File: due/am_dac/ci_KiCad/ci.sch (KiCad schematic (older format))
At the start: 8 parts

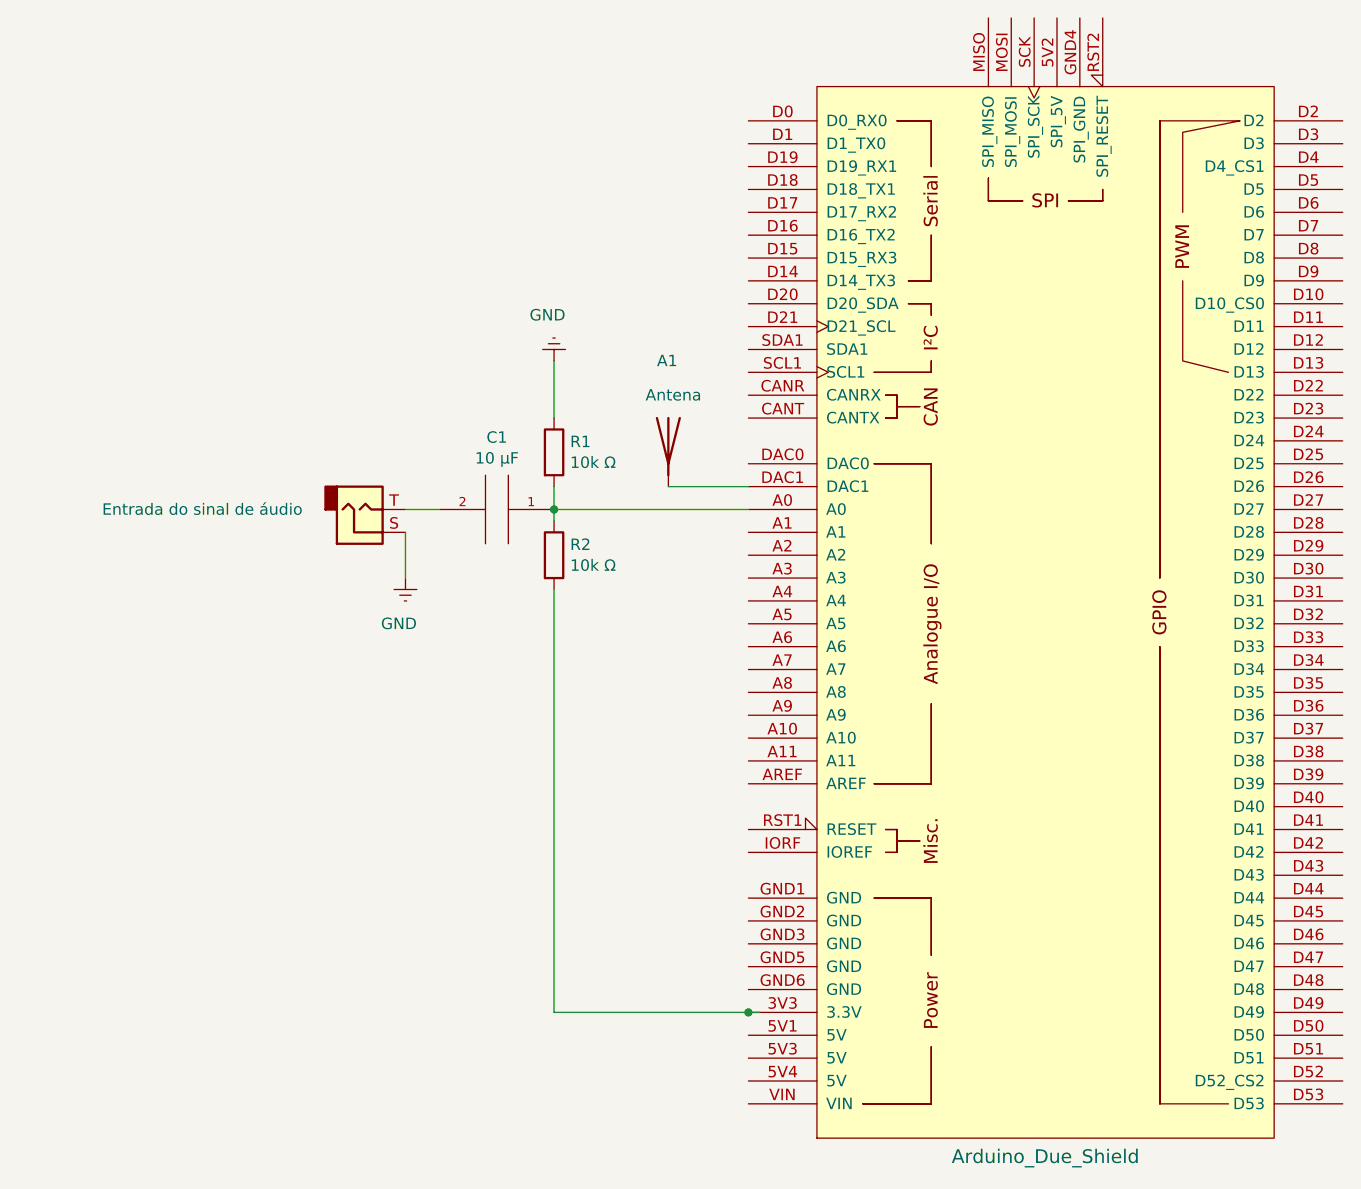
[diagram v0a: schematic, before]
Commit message: Update due am_dac project
Signed-off-by: fgl27 <fglfgl27@gmail.com>
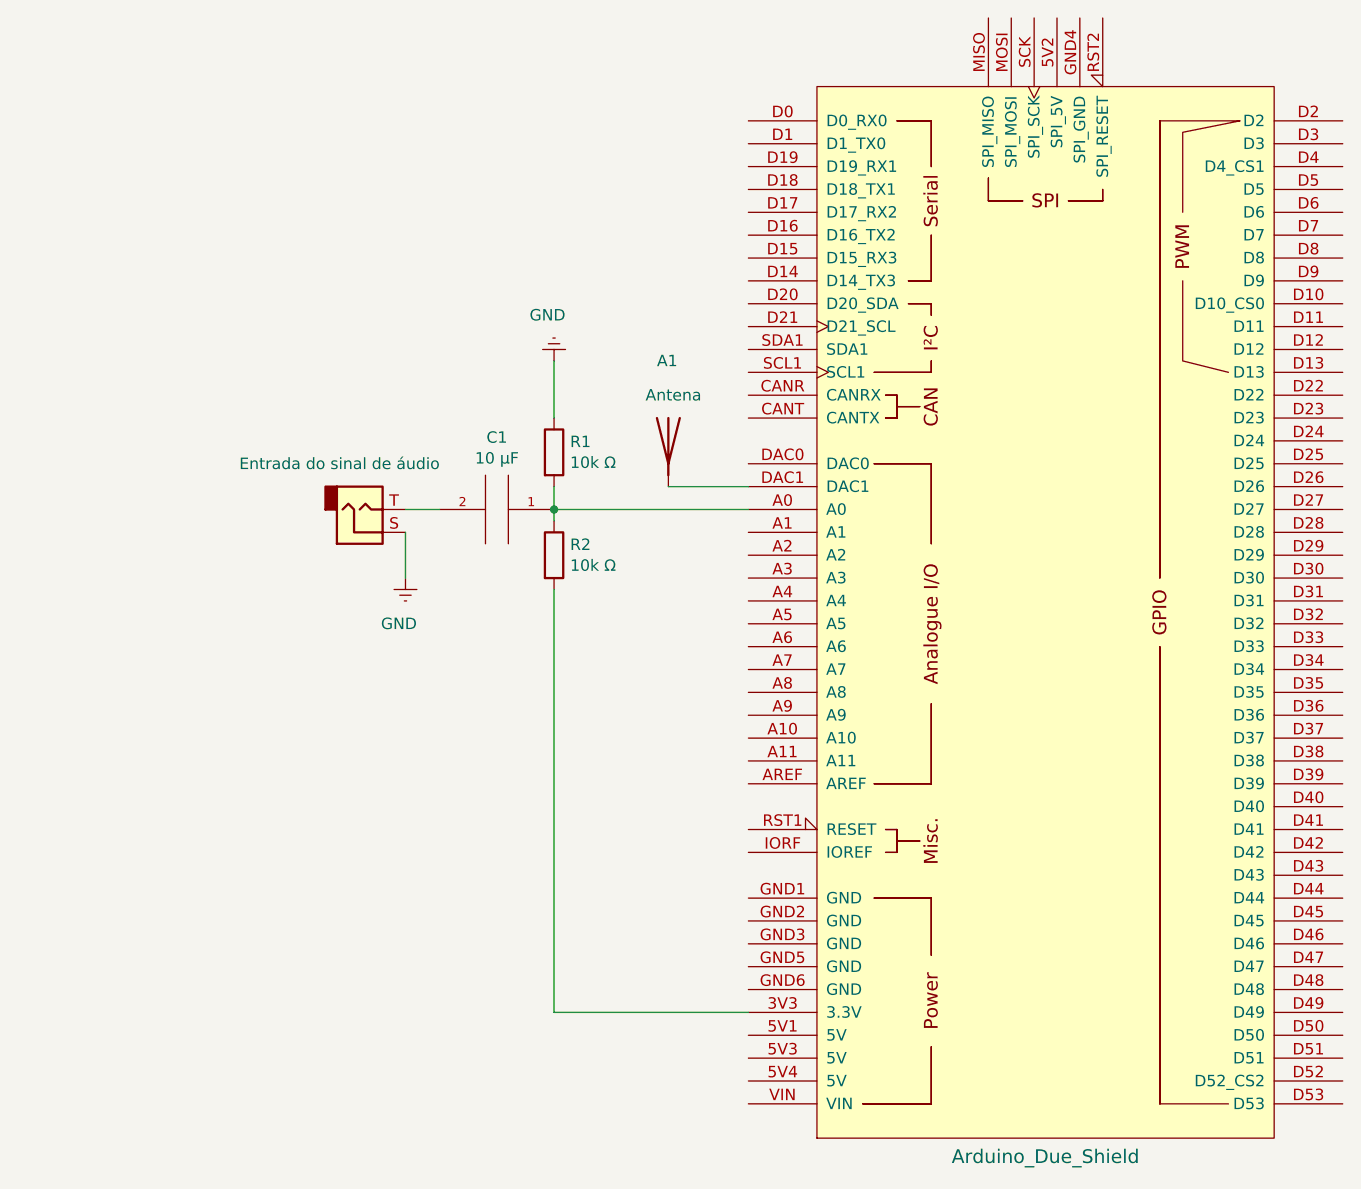
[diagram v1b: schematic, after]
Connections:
- wire segments 10 -> 9
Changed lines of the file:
@@
 P 2600 3250
 F 0 "J?" V 2678 3120 50  0001 R CNN
-F 1 "Entrada do sinal de áudio" H 2350 3250 50  0000 R CNN
+F 1 "Entrada do sinal de áudio" H 2950 3050 50  0000 R CNN
 F 2 "" H 2600 3250 50  0001 C CNN
 F 3 "~" H 2600 3250 50  0001 C CNN
@@
 Wire Wire Line
 	3450 2850 3450 2600
+Wire Wire Line
+	3950 3150 4300 3150
+Wire Wire Line
+	3450 5450 3450 3600
+Wire Wire Line
+	3450 3250 4300 3250
 $Comp
 L arduino:Arduino_Due_Shield XA1
@@
 $EndComp
 Wire Wire Line
-	3950 3150 4300 3150
-Wire Wire Line
-	3450 3250 4300 3250
-Wire Wire Line
-	4350 5450 4300 5450
-Wire Wire Line
-	3450 5450 3450 3600
-Connection ~ 4300 5450
-Wire Wire Line
 	4300 5450 3450 5450

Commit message: Up due am_dac
Signed-off-by: fgl27 <fglfgl27@gmail.com>
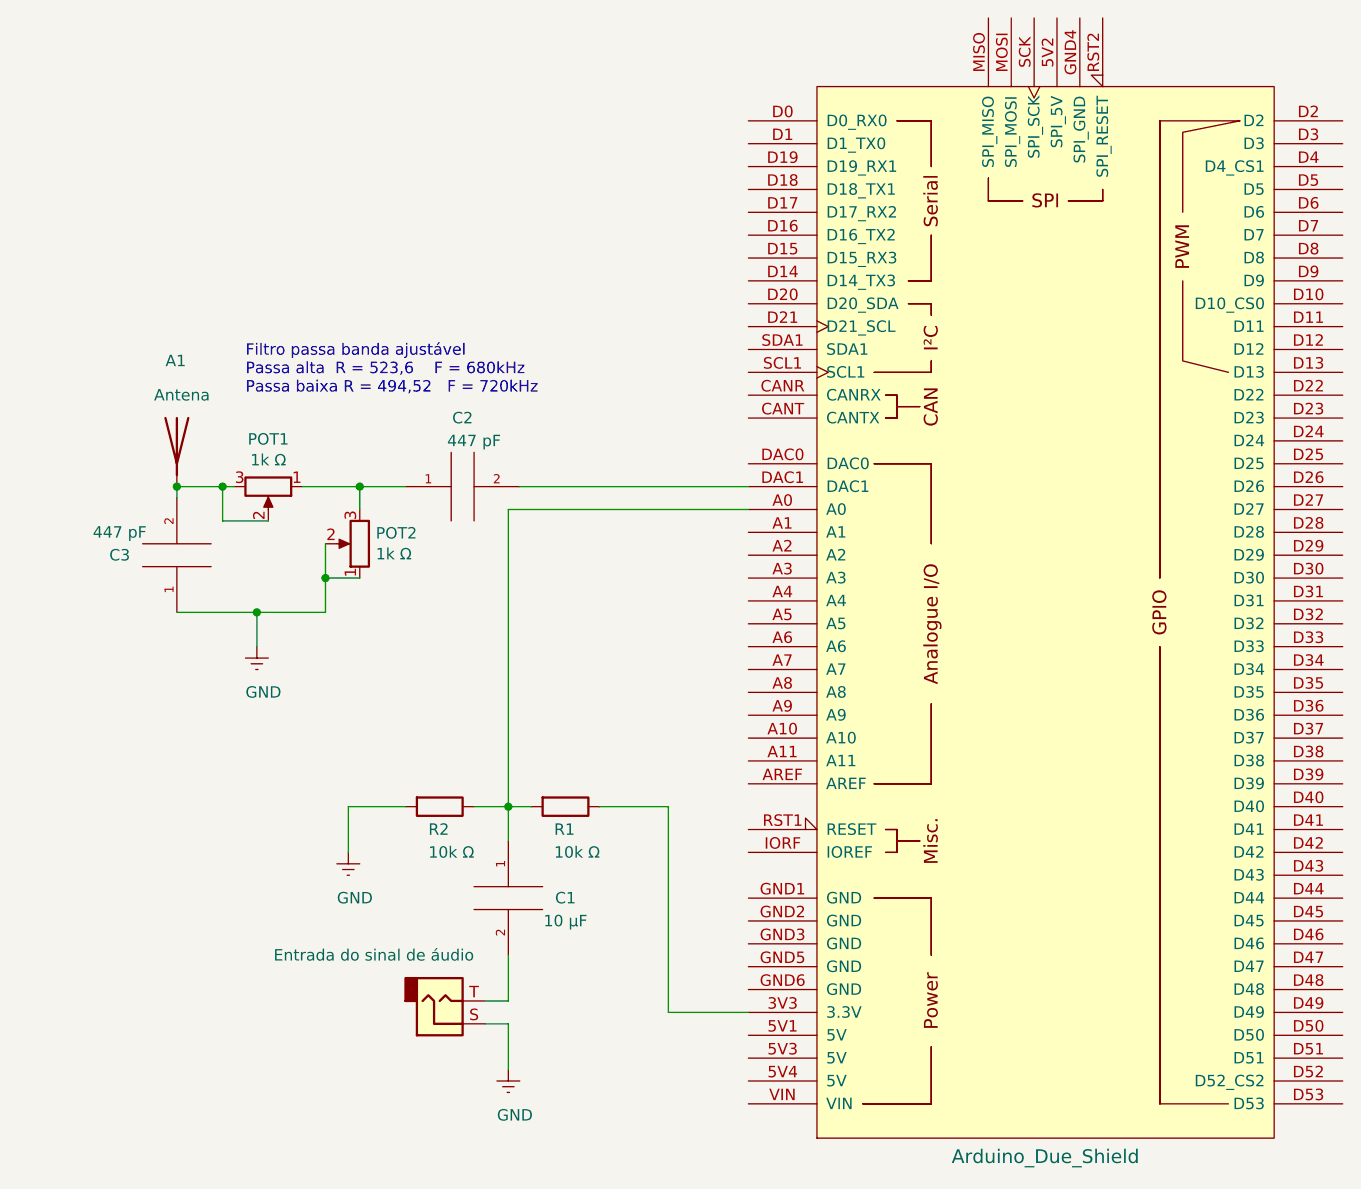
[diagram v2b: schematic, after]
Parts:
- removed GND: GNDREF, symbol power:GNDREF
- added C2, C3: 447 pF, symbol pspice:CAP
- added GND (x2): GNDREF, symbol power:GNDREF
- added POT1, POT2: 1k Ω, symbol Device:R_POT
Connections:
- net GNDREF: now also R2.2, C3.1, GND.1 (GNDREF), GND.1 (GNDREF), POT2.1, POT2.2; no longer R1.1
- net at A1.1 (A): now also C3.2, POT1.2, POT1.3; no longer XA1.DAC1
- net at XA1.3V3 (3.3V): now also R1.1; no longer R2.2
- new net: C2.2, XA1.DAC1
- new net: C2.1, POT1.1, POT2.3
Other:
- note added: "Filtro passa banda ajustável\nPassa alta R = 523,6 F = 680kHz\nPassa baixa R = 494,52 F = 720kHz"
- moved on the sheet: A1, C1, R1, R2
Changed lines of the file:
@@
 L Device:Antenna A1
 U 1 1 605397BD
-P 3950 2950
-F 0 "A1" H 3900 3300 50  0000 L CNN
-F 1 "Antena" H 3850 3150 50  0000 L CNN
-F 2 "" H 3950 2950 50  0001 C CNN
-F 3 "~" H 3950 2950 50  0001 C CNN
-	1    3950 2950
+P 1800 2950
+F 0 "A1" H 1750 3300 50  0000 L CNN
+F 1 "Antena" H 1700 3150 50  0000 L CNN
+F 2 "" H 1800 2950 50  0001 C CNN
+F 3 "~" H 1800 2950 50  0001 C CNN
+	1    1800 2950
 	1    0    0    -1
 $EndComp
@@
 L Device:R R1
 U 1 1 6053A6BF
-P 3450 3000
-F 0 "R1" H 3520 3046 50  0000 L CNN
-F 1 "10k Ω" H 3520 2955 50  0000 L CNN
-F 2 "" V 3380 3000 50  0001 C CNN
-F 3 "~" H 3450 3000 50  0001 C CNN
-	1    3450 3000
-	1    0    0    -1
+P 3500 4550
+F 0 "R1" V 3600 4500 50  0000 L CNN
+F 1 "10k Ω" V 3700 4500 50  0000 L CNN
+F 2 "" V 3430 4550 50  0001 C CNN
+F 3 "~" H 3500 4550 50  0001 C CNN
+	1    3500 4550
+	0    1    1    0
 $EndComp
 $Comp
 L pspice:CAP C1
 U 1 1 6053AEF6
-P 3200 3250
-F 0 "C1" V 3515 3250 50  0000 C CNN
-F 1 "10 μF" V 3424 3250 50  0000 C CNN
-F 2 "" H 3200 3250 50  0001 C CNN
-F 3 "~" H 3200 3250 50  0001 C CNN
-	1    3200 3250
-	0    1    -1   0
+P 3250 4950
+F 0 "C1" H 3000 4950 50  0000 C CNN
+F 1 "10 μF" H 3000 4850 50  0000 C CNN
+F 2 "" H 3250 4950 50  0001 C CNN
+F 3 "~" H 3250 4950 50  0001 C CNN
+	1    3250 4950
+	-1   0    0    -1
 $EndComp
 $Comp
 L Connector:AudioJack2 J?
 U 1 1 6053CCAD
-P 2600 3250
-F 0 "J?" V 2678 3120 50  0001 R CNN
-F 1 "Entrada do sinal de áudio" H 2950 3050 50  0000 R CNN
-F 2 "" H 2600 3250 50  0001 C CNN
-F 3 "~" H 2600 3250 50  0001 C CNN
-	1    2600 3250
+P 2950 5400
+F 0 "J?" V 3028 5270 50  0001 R CNN
+F 1 "Entrada do sinal de áudio" H 3100 5200 50  0000 R CNN
+F 2 "" H 2950 5400 50  0001 C CNN
+F 3 "~" H 2950 5400 50  0001 C CNN
+	1    2950 5400
 	1    0    0    1
 $EndComp
@@
 L Device:R R2
 U 1 1 6053E3D1
-P 3450 3450
-F 0 "R2" H 3520 3496 50  0000 L CNN
-F 1 "10k Ω" H 3520 3405 50  0000 L CNN
-F 2 "" V 3380 3450 50  0001 C CNN
-F 3 "~" H 3450 3450 50  0001 C CNN
-	1    3450 3450
-	1    0    0    -1
-$EndComp
-Wire Wire Line
-	3450 3150 3450 3250
-Connection ~ 3450 3250
-Wire Wire Line
-	3450 3250 3450 3300
-Wire Wire Line
-	2800 3250 2950 3250
-$Comp
-L power:GNDREF GND
-U 1 1 605473BE
-P 2800 3550
-F 0 "GND" H 2750 3350 50  0000 L CNN
-F 1 "GNDREF" H 2805 3377 50  0001 C CNN
-F 2 "" H 2800 3550 50  0001 C CNN
-F 3 "" H 2800 3550 50  0001 C CNN
-	1    2800 3550
-	-1   0    0    -1
-$EndComp
-Wire Wire Line
-	2800 3550 2800 3350
+P 2950 4550
+F 0 "R2" V 3050 4500 50  0000 L CNN
+F 1 "10k Ω" V 3150 4500 50  0000 L CNN
+F 2 "" V 2880 4550 50  0001 C CNN
+F 3 "~" H 2950 4550 50  0001 C CNN
+	1    2950 4550
+	0    1    1    0
+$EndComp
 $Comp
 L power:GNDREF GND
 U 1 1 60554C55
-P 3450 2600
-F 0 "GND" H 3400 2400 50  0000 L CNN
-F 1 "GNDREF" H 3455 2427 50  0001 C CNN
-F 2 "" H 3450 2600 50  0001 C CNN
-F 3 "" H 3450 2600 50  0001 C CNN
-	1    3450 2600
-	-1   0    0    1
-$EndComp
-Wire Wire Line
-	3450 2850 3450 2600
-Wire Wire Line
-	3950 3150 4300 3150
-Wire Wire Line
-	3450 5450 3450 3600
-Wire Wire Line
-	3450 3250 4300 3250
+P 2550 4750
+F 0 "GND" H 2500 4550 50  0000 L CNN
+F 1 "GNDREF" H 2555 4577 50  0001 C CNN
+F 2 "" H 2550 4750 50  0001 C CNN
+F 3 "" H 2550 4750 50  0001 C CNN
+	1    2550 4750
+	1    0    0    -1
+$EndComp
 $Comp
 L arduino:Arduino_Due_Shield XA1
@@
 	1    0    0    -1
 $EndComp
-Wire Wire Line
-	4300 5450 3450 5450
+$Comp
+L Device:R_POT POT2
+U 1 1 60927CF1
+P 2600 3400
+F 0 "POT2" H 2530 3354 50  0000 R CNN
+F 1 "1k Ω" H 2530 3445 50  0000 R CNN
+F 2 "" H 2600 3400 50  0001 C CNN
+F 3 "~" H 2600 3400 50  0001 C CNN
+	1    2600 3400
+	-1   0    0    1
+$EndComp
+Wire Wire Line
+	3350 4550 3250 4550
+Wire Wire Line
+	2800 4550 2550 4550
+Wire Wire Line
+	2550 4550 2550 4750
+Wire Wire Line
+	3150 5400 3250 5400
+Wire Wire Line
+	3250 5400 3250 5200
+Wire Wire Line
+	3250 5500 3250 5700
+$Comp
+L power:GNDREF GND
+U 1 1 60962530
+P 3250 5700
+F 0 "GND" H 3200 5500 50  0000 L CNN
+F 1 "GNDREF" H 3255 5527 50  0001 C CNN
+F 2 "" H 3250 5700 50  0001 C CNN
+F 3 "" H 3250 5700 50  0001 C CNN
+	1    3250 5700
+	1    0    0    -1
+$EndComp
+Wire Wire Line
+	3150 5500 3250 5500
+Wire Wire Line
+	3250 4700 3250 4550
+Connection ~ 3250 4550
+Wire Wire Line
+	3250 4550 3100 4550
+$Comp
+L pspice:CAP C2
+U 1 1 6097110B
+P 3050 3150
+F 0 "C2" V 2750 3150 50  0000 C CNN
+F 1 "447 pF" V 2850 3100 50  0000 C CNN
+F 2 "" H 3050 3150 50  0001 C CNN
+F 3 "~" H 3050 3150 50  0001 C CNN
+	1    3050 3150
+	0    -1   1    0
+$EndComp
+$Comp
+L Device:R_POT POT1
+U 1 1 60975627
+P 2200 3150
+F 0 "POT1" V 1993 3150 50  0000 C CNN
+F 1 "1k Ω" V 2084 3150 50  0000 C CNN
+F 2 "" H 2200 3150 50  0001 C CNN
+F 3 "~" H 2200 3150 50  0001 C CNN
+	1    2200 3150
+	0    1    1    0
+$EndComp
+$Comp
+L pspice:CAP C3
+U 1 1 60979D61
+P 1800 3450
+F 0 "C3" H 1550 3450 50  0000 C CNN
+F 1 "447 pF" H 1550 3350 50  0000 C CNN
+F 2 "" H 1800 3450 50  0001 C CNN
+F 3 "~" H 1800 3450 50  0001 C CNN
+	1    1800 3450
+	1    0    0    1
+$EndComp
+$Comp
+L power:GNDREF GND
+U 1 1 6097D7CE
+P 2150 3850
+F 0 "GND" H 2100 3650 50  0000 L CNN
+F 1 "GNDREF" H 2155 3677 50  0001 C CNN
+F 2 "" H 2150 3850 50  0001 C CNN
+F 3 "" H 2150 3850 50  0001 C CNN
+	1    2150 3850
+	1    0    0    -1
+$EndComp
+Wire Wire Line
+	3300 3150 4300 3150
+Wire Wire Line
+	2800 3150 2600 3150
+Wire Wire Line
+	2600 3250 2600 3150
+Connection ~ 2600 3150
+Wire Wire Line
+	2600 3150 2350 3150
+Wire Wire Line
+	1800 3200 1800 3150
+Wire Wire Line
+	1800 3150 2000 3150
+Wire Wire Line
+	2450 3400 2450 3550
+Wire Wire Line
+	2150 3850 2150 3700
+Wire Wire Line
+	1800 3700 2150 3700
+Connection ~ 2150 3700
+Wire Wire Line
+	2150 3700 2450 3700
+Connection ~ 1800 3150
+Wire Wire Line
+	2600 3550 2450 3550
+Connection ~ 2450 3550
+Wire Wire Line
+	2450 3550 2450 3700
+Wire Wire Line
+	2200 3300 2000 3300
+Wire Wire Line
+	2000 3300 2000 3150
+Connection ~ 2000 3150
+Wire Wire Line
+	2000 3150 2050 3150
+Wire Wire Line
+	4300 5450 3950 5450
+Wire Wire Line
+	3950 5450 3950 4550
+Wire Wire Line
+	3950 4550 3650 4550
+Wire Wire Line
+	3250 4550 3250 3250
+Wire Wire Line
+	3250 3250 4300 3250
+Text Notes 2100 2750 0    50   ~ 0
+Filtro passa banda ajustável\nPassa alta  R = 523,6    F = 680kHz\nPassa baixa R = 494,52   F = 720kHz
 $EndSCHEMATC
